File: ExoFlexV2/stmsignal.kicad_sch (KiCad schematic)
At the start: 4 parts, among them J4 CN9, J5 CN8, J6 CN7, J7 CN10

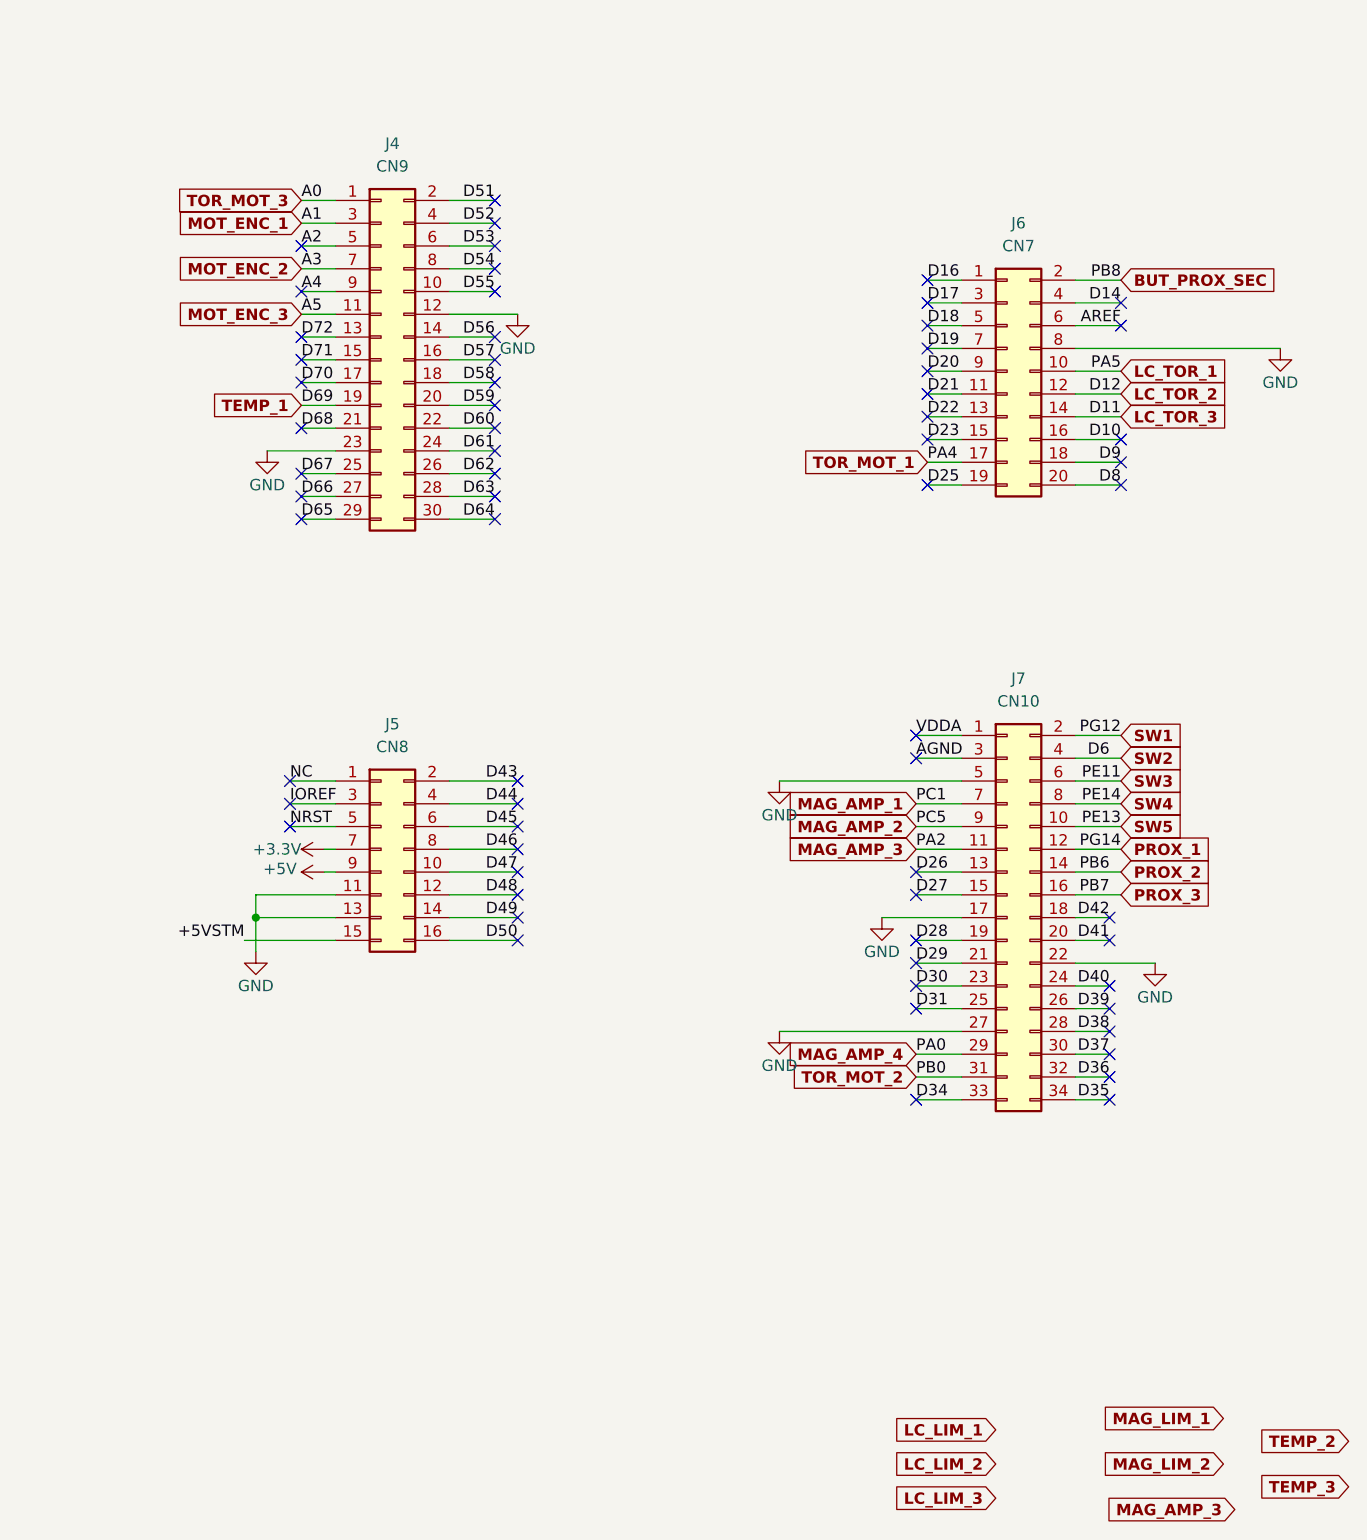
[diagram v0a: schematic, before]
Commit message: Placement
Début du placement et modification d'après dernier review
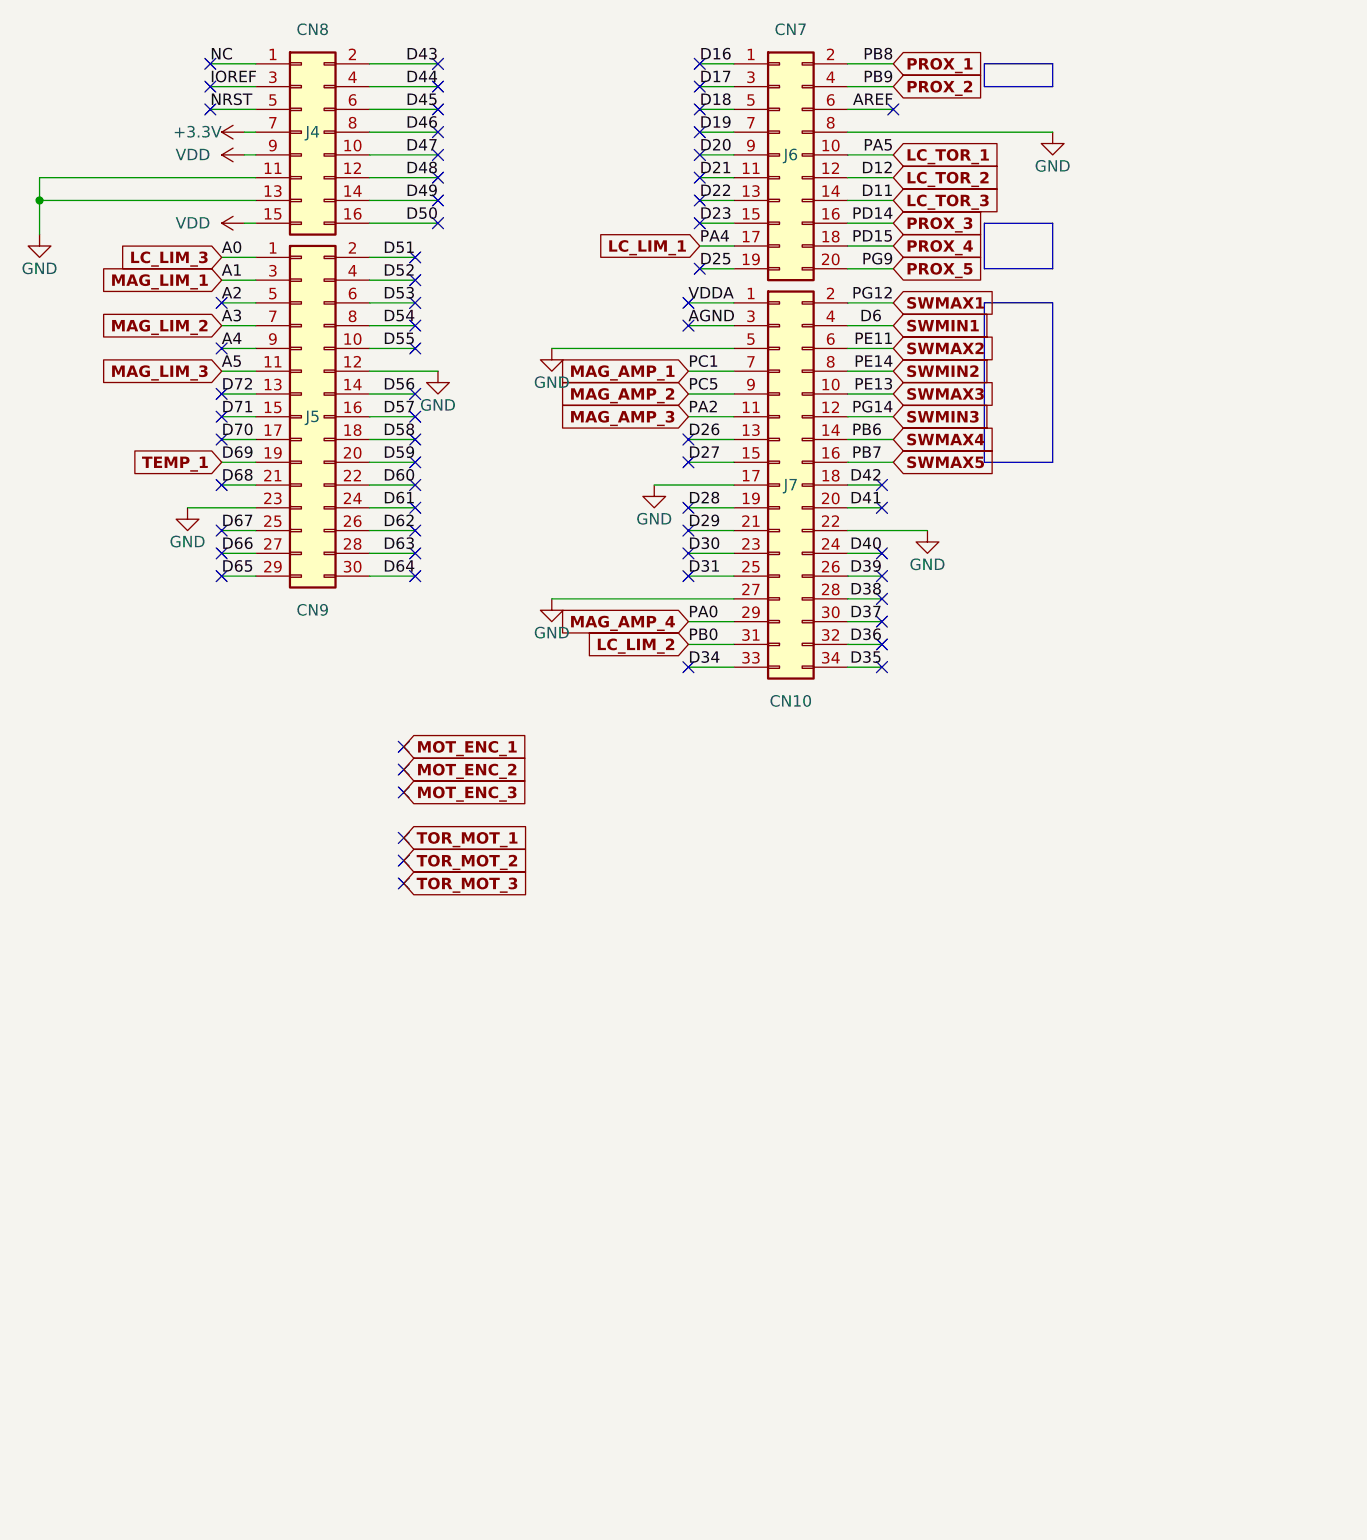
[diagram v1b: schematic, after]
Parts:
- renumbered J5 to J4, J4 to J5
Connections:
- net +5VSTM is gone; now on net VDD: J4.15 (Pin_15)
- net BUT_PROX_SEC is gone; now on net PROX_1: J6.2 (Pin_2)
- net D10 is gone; now on net PROX_3: J6.16 (Pin_16)
- net D14 is gone; now on net PROX_2: J6.4 (Pin_4)
- net LC_LIM_1: now also J6.17 (Pin_17)
- net LC_LIM_2: now also J7.31 (Pin_31)
- net LC_LIM_3: now also J5.1 (Pin_1)
- net MAG_LIM_1: now also J5.3 (Pin_3)
- net MAG_LIM_2: now also J5.7 (Pin_7)
- net MOT_ENC_1: no longer J5.3 (Pin_3)
- net MOT_ENC_2: no longer J5.7 (Pin_7)
- net MOT_ENC_3: no longer J5.11 (Pin_11)
- net PROX_1: no longer J7.12 (Pin_12)
- net PROX_2: no longer J7.14 (Pin_14)
- net PROX_3: no longer J7.16 (Pin_16)
- net TOR_MOT_1: no longer J6.17 (Pin_17)
- net TOR_MOT_2: no longer J7.31 (Pin_31)
- net TOR_MOT_3: no longer J5.1 (Pin_1)
- net +5V renamed VDD
- net D8 renamed PROX_5
- net D9 renamed PROX_4
- net SW1 renamed SWMAX1
- net SW2 renamed SWMIN1
- net SW3 renamed SWMAX2
- net SW4 renamed SWMIN2
- net SW5 renamed SWMAX3
- new net MAG_LIM_3: J5.11 (Pin_11)
- new net SWMAX4: J7.14 (Pin_14)
- new net SWMAX5: J7.16 (Pin_16)
- new net SWMIN3: J7.12 (Pin_12)
- no-connect marks 65 -> 67
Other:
- moved on the sheet: J4, J5, J6, J7
